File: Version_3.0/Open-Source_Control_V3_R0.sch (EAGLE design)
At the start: 349 parts, among them IC10 MCP6002SMT, IC11 MCP6002SMT, IC12 MCP6002SMT, IC14 MCP6002SMT, IC2 ULN2003AD, IC4 74HC165D, IC5 74HC165D, J24 6p-2.54, K1 G5LE-14-CF DC24, K2 G5LE-14-CF DC24, K3 G5LE-14-CF DC24, K4 G5LE-14-CF DC24, Q1 MMBT2907, T4 DA2304-AL, U1 OSD3358-512M-ICB, U16 AT97SC3205T-G3M4400B, U2 TPD4S012_DRY_6_P1_M, U27 LAN8710, U28 TCAN1051HV, U29 MAX3483EESA+T, U4 APX811-31UGSOT, U40 ISO3086TDW, U5 TLVH431, U6 SN74LVC2G241_DCU_8, X1 10118194-0001LF, X10 MC4, X11 MC4, X12 MC4, X2 J0011D01BNL, X21 MC12, X24 MSTBA2, X3 MC4, X31 MC4, X4 CTI-JTAG, X41 MSTBA3, X5 DM3CS-SF, X6 6p-2.54, X7 TH-2X10, X8 TH-2X10, X9 5600200420, Y7 ECS-250-12-30-GN-TR

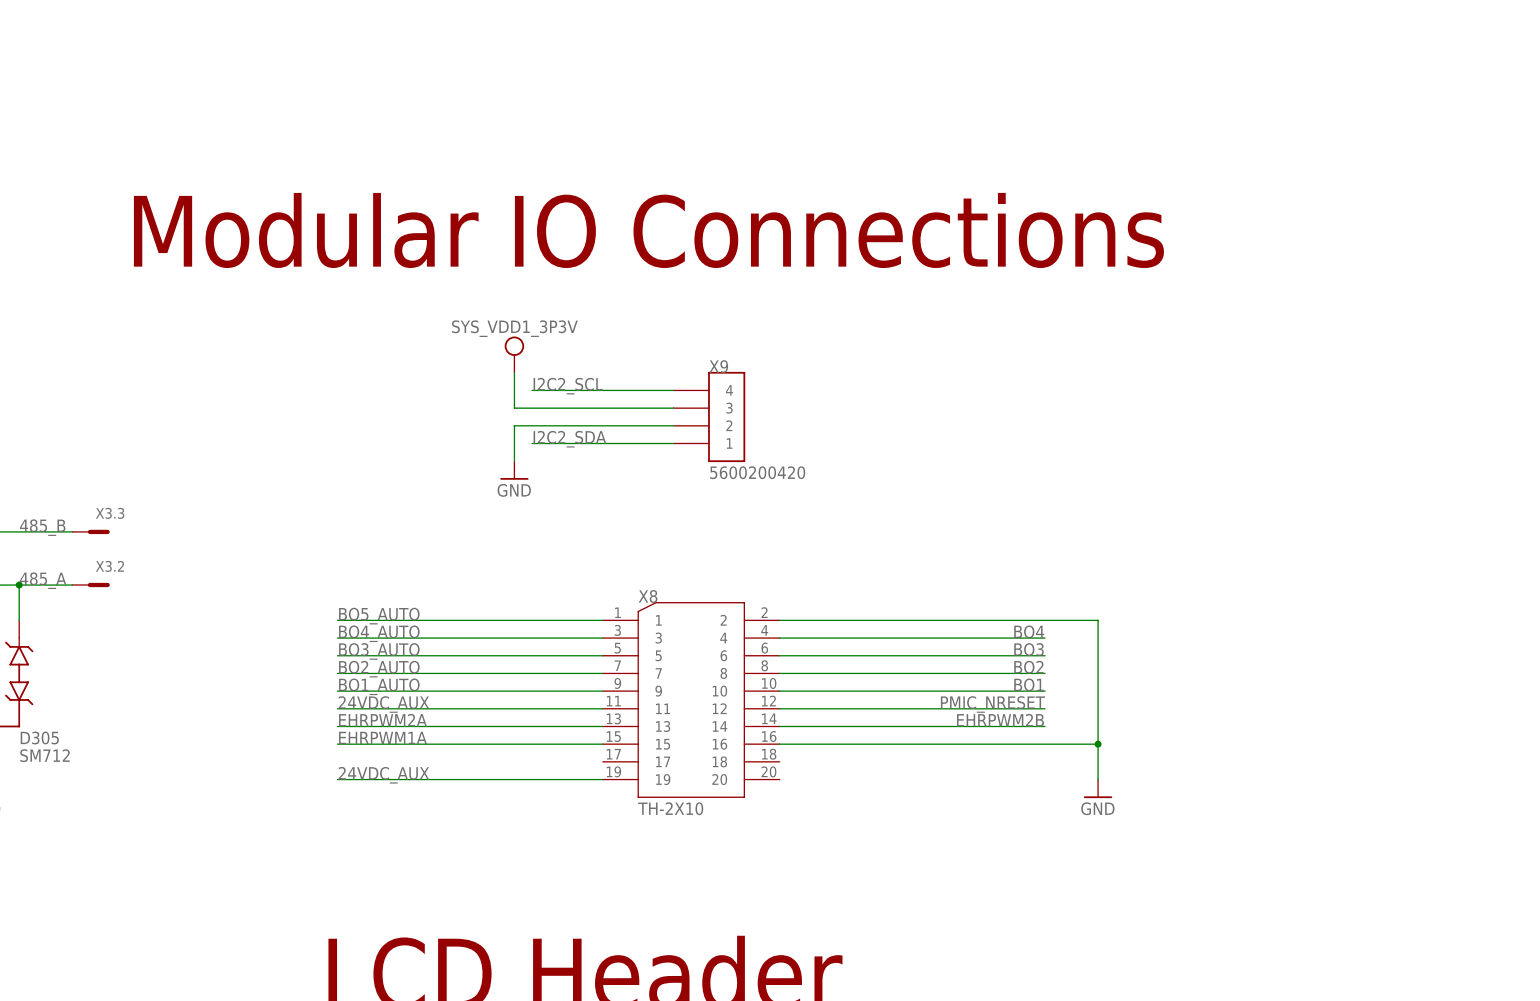
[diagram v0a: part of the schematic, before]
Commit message: Add files via upload
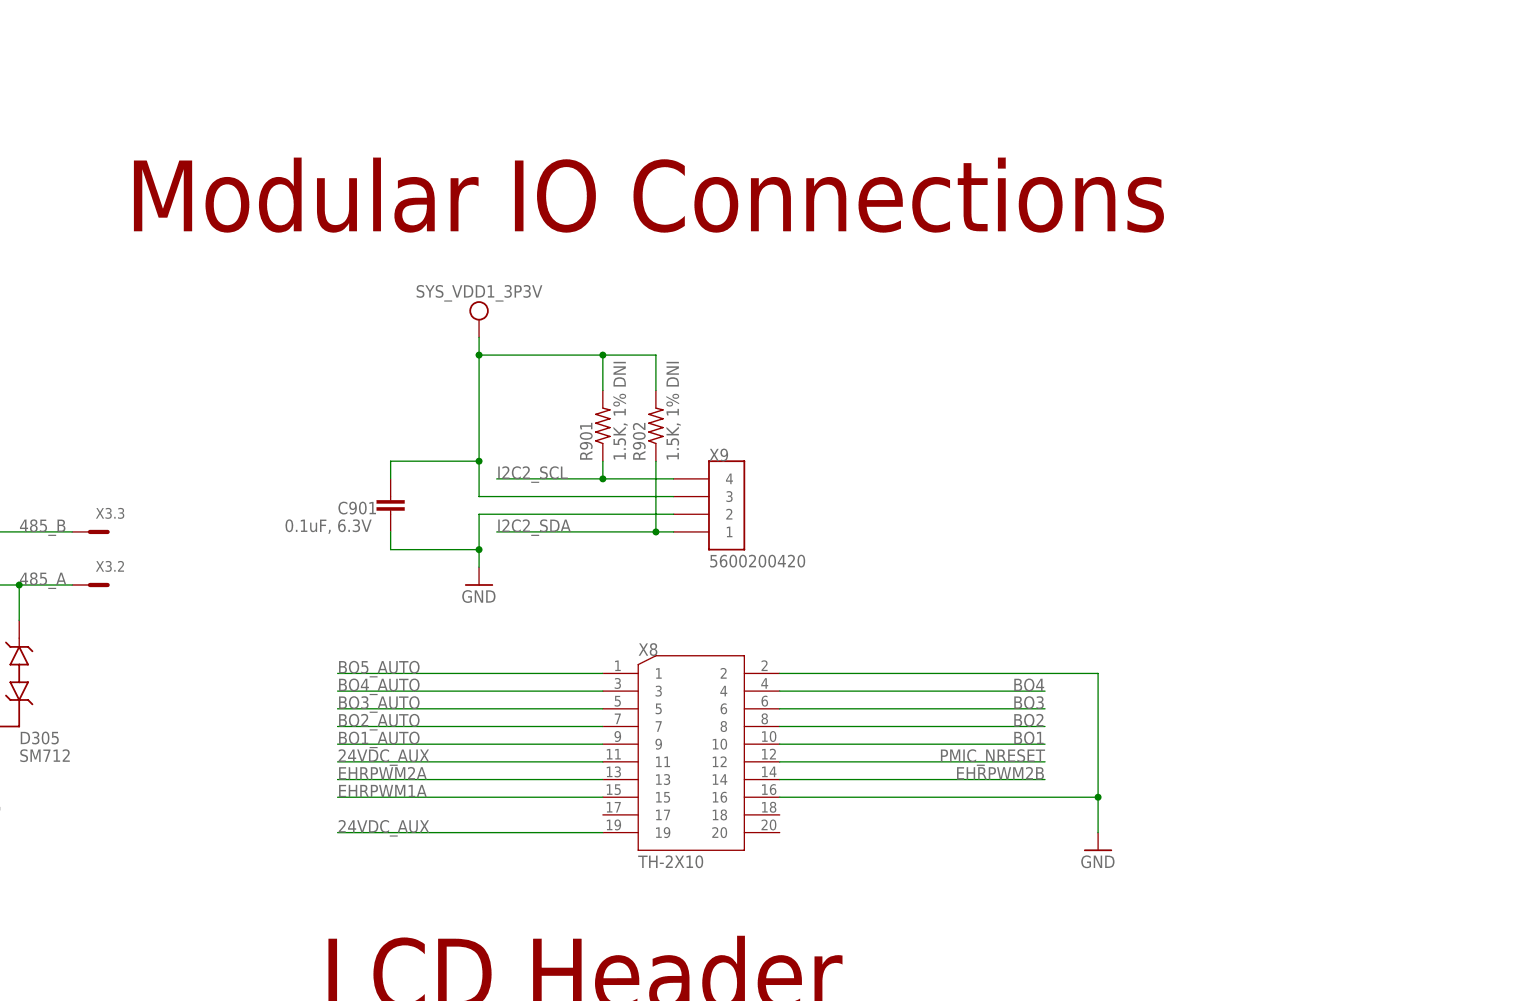
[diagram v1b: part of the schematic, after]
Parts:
- added C901: 0.1uF, 6.3V, OSD3358-SM-RED Platform:CC0402
- added R901, R902: 1.5K, 1% DNI, OSD3358-SM-RED Platform:R-US_R0402
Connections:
- net GND: now also C901.2
- net I2C2_SCL: now also R901.1
- net I2C2_SDA: now also R902.1
- net SYS_VDD1_3P3V: now also C901.1, R901.2, R902.2
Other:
- note added: "Airflow Sensor Conn"
- moved on the sheet: X8, X9
